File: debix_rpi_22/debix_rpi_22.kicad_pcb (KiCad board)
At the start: 2 copper layers, 71 x 12.5 mm, 2 parts, among them J1 Conn_01x24, J3 RPi 22 Pin MIPI CSI-2

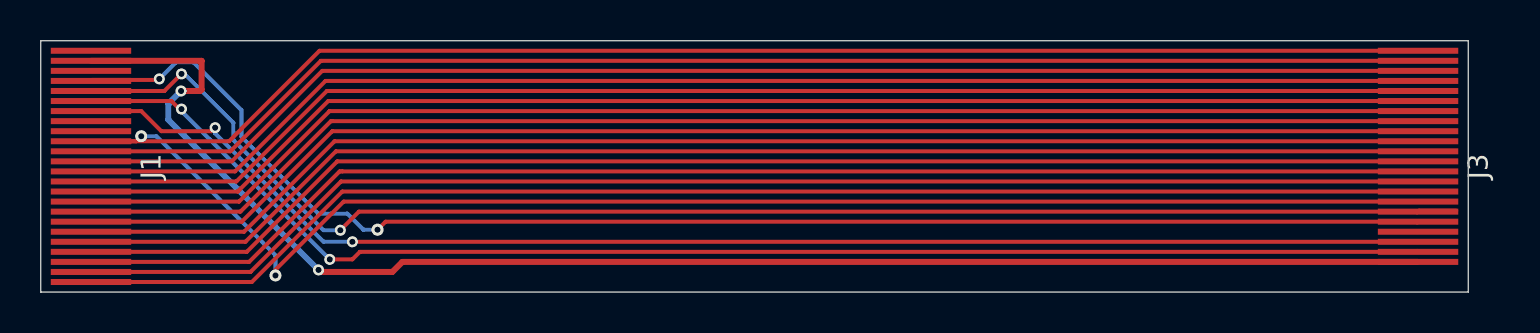
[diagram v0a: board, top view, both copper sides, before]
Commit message: rounded tracks...
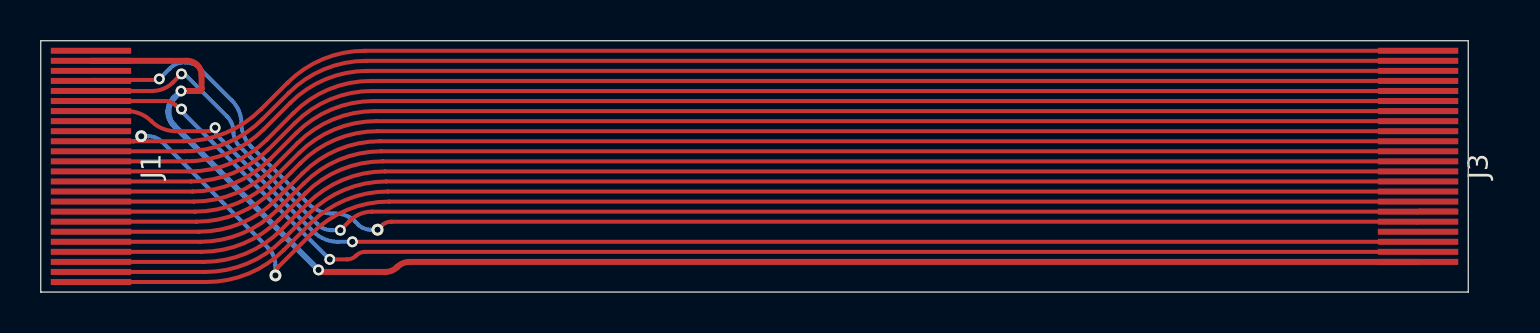
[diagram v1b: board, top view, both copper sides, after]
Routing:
- net GND: track 408.6 -> 405.7 mm
- net +3V3: track 75.2 -> 74.6 mm
- net /CAM_GPIO_1: track 70.8 -> 70.3 mm
- net /csi_d3_P: track 67.9 -> 67.3 mm
- net /csi_d3_N: track 67.9 -> 67.3 mm
- net /csi_d2_P: track 67.9 -> 67.3 mm
- net /csi_clk_N: track 67.9 -> 67.3 mm
- net /csi_d2_N: track 67.9 -> 67.3 mm
- net /csi_d1_N: track 67.9 -> 67.3 mm
- net /csi_d0_P: track 67.9 -> 67.3 mm
- net /csi_d0_N: track 67.9 -> 67.3 mm
- net /csi_clk_P: track 67.9 -> 67.3 mm
- net /csi_d1_P: track 67.9 -> 67.3 mm
